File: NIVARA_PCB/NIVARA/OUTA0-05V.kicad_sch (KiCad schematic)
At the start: 0 parts

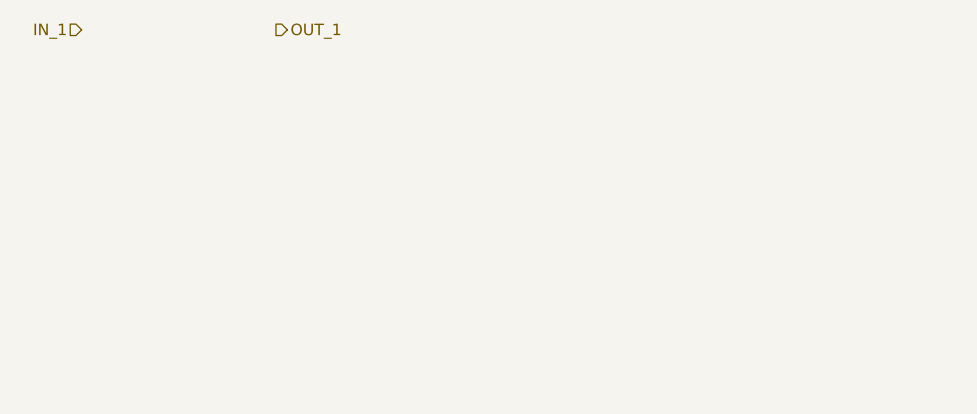
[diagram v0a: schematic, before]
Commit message: SALIDAS DE VOLTAJE Y CORRIENTE
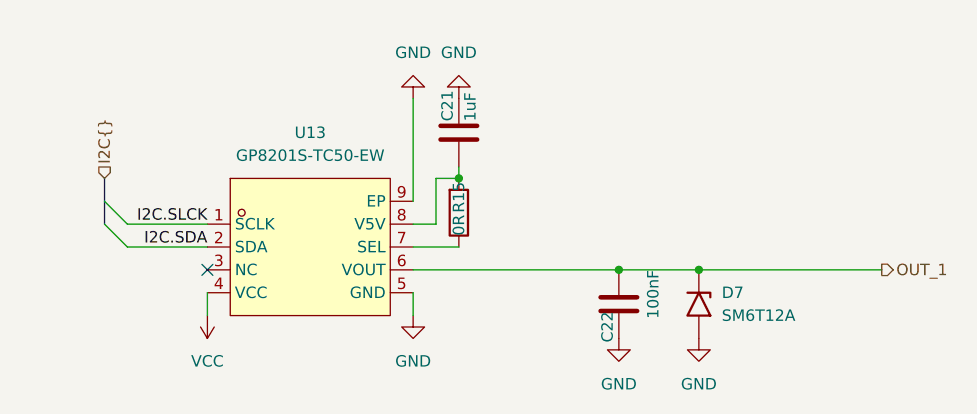
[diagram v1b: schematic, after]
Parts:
- added C21: 1uF, PCM_Capacitor_SMD_AKL:C_0603_1608Metric, symbol PCM_Capacitor_AKL:C_0603
- added C22: 100nF, PCM_Capacitor_SMD_AKL:C_0603_1608Metric, symbol PCM_Capacitor_AKL:C_0603
- added D7: SM6T12A, Diode_SMD:D_SMB, symbol Diode:SM6T12A
- added R15: 0R, PCM_Resistor_SMD_AKL:R_0603_1608Metric, symbol PCM_Resistor_AKL:R_0603
- added U13: GP8201S-TC50-EW, easyeda2kicad:ESOP-8_L4.9-W3.9-P1.27-LS6.0-BL-EP, symbol easyeda2kicad:GP8201S-TC50-EW
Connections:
- net OUT_1: now also C22.2, D7.1 (A1), U13.6 (VOUT)
- new net: C21.2, R15.1, U13.8 (V5V)
- new net: R15.2, U13.7 (SEL)
- new net GND: C21.1, C22.1, D7.2 (A2), U13.5 (GND), U13.9 (EP)
- new net I2C.SDA: U13.2 (SDA)
- new net I2C.SLCK: U13.1 (SCLK)
- new net VCC: U13.4 (VCC)
- no-connect marks 0 -> 1

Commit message: ACTUALIZACION
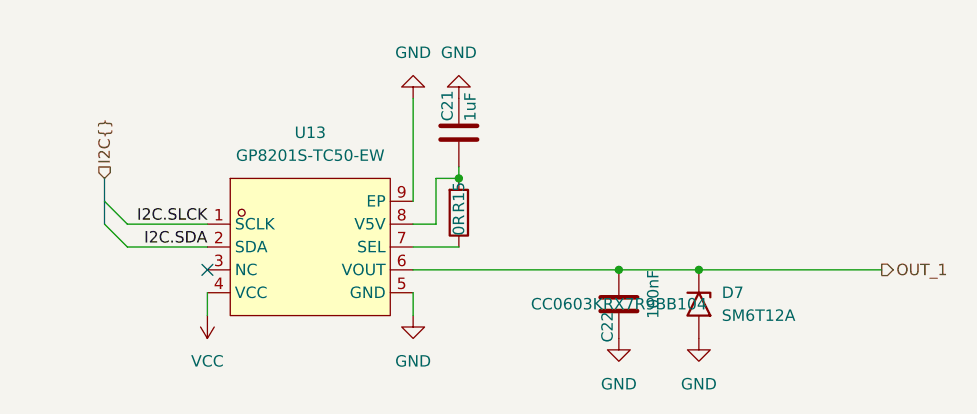
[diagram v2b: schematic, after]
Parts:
- C22: PART NUMBERT (none) -> CC0603KRX7R9BB104
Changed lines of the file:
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@@
 			)
 		)
-		(property "PART NUMBERT" ""
+		(property "PART NUMBERT" "CC0603KRX7R9BB104"
 			(at 93.98 60.96 0)
 			(effects
